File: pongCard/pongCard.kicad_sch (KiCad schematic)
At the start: 25 parts, among them J1 USB_B_Micro, J2 Conn_02x04_Odd_Even, J3 Conn_02x04_Odd_Even, U1 ESP-01v090, U2 HT75xx-1-SOT89, U3 ESP-12E

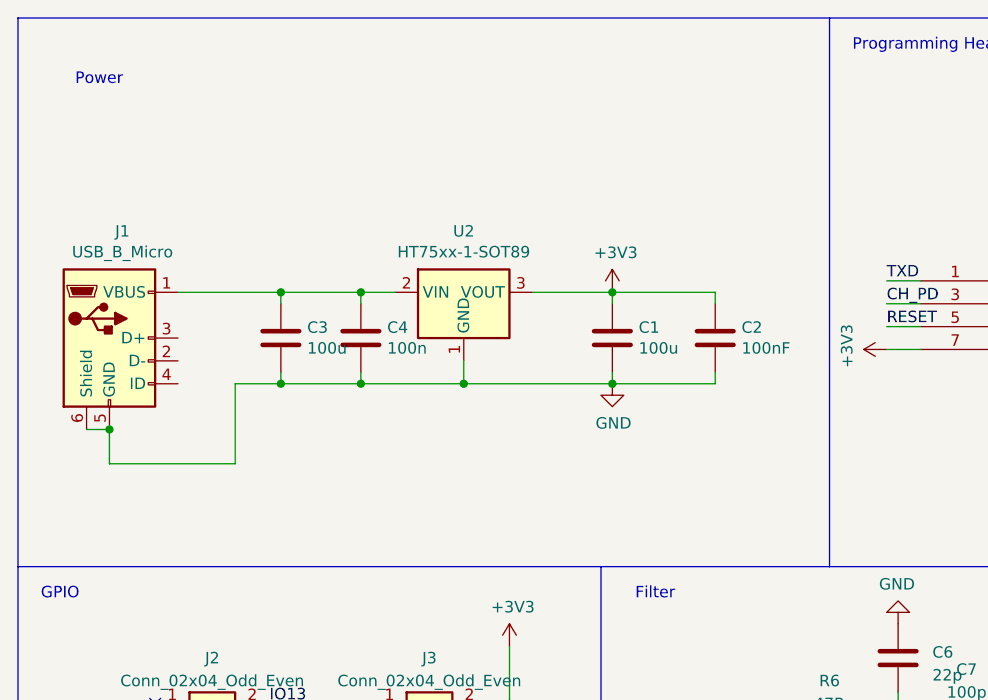
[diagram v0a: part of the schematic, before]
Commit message: V3: Battery Step up
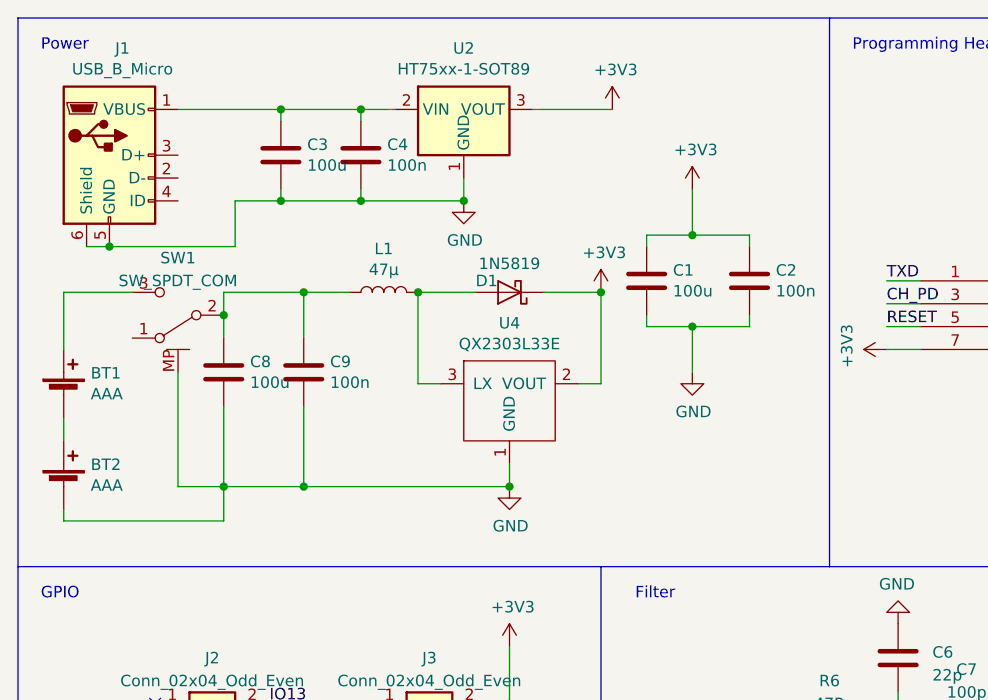
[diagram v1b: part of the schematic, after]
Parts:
- added BT1, BT2: AAA, pongCard:BatteryHolder_AAA_MYOUNG, symbol hh2020v1-rescue:Battery_Cell-Device
- added C8: 100u, Capacitor_SMD:C_1206_3216Metric_Pad1.33x1.80mm_HandSolder, symbol Device:C
- added C9: 100n, Capacitor_SMD:C_0603_1608Metric_Pad1.08x0.95mm_HandSolder, symbol Device:C
- added D1: 1N5819, Diode_SMD:D_SOD-123, symbol hh2020v1-rescue:1N5819-Diode
- added L1: 47µ, Inductor_SMD:L_1210_3225Metric_Pad1.42x2.65mm_HandSolder, symbol hh2020v1-rescue:L-Device
- added SW1: SW_SPDT_COM, pongCard:SW_SPDT_PCM12_COM, symbol pongCard:SW_SPDT_COM
- added U4: QX2303L33E, Package_TO_SOT_SMD:SOT-89-3_Handsoldering, symbol QX2303L33E:QX2303L33E
- C2: value 100nF -> 100n
- U2: footprint Package_TO_SOT_SMD:SOT-89-3 -> Package_TO_SOT_SMD:SOT-89-3_Handsoldering
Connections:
- net +3V3: now also D1.1 (K), U4.2 (VOUT)
- net GND: now also BT2.2 (-), C8.2, C9.2, SW1.MP, U4.1 (GND)
- new net: BT1.1 (+), SW1.3 (C)
- new net: BT1.2 (-), BT2.1 (+)
- new net: C8.1, C9.1, L1.1, SW1.2 (B)
- new net: D1.2 (A), L1.2, U4.3 (LX)
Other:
- moved on the sheet: C3, C4, J1, U2
